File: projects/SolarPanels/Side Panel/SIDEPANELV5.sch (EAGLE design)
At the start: 31 parts

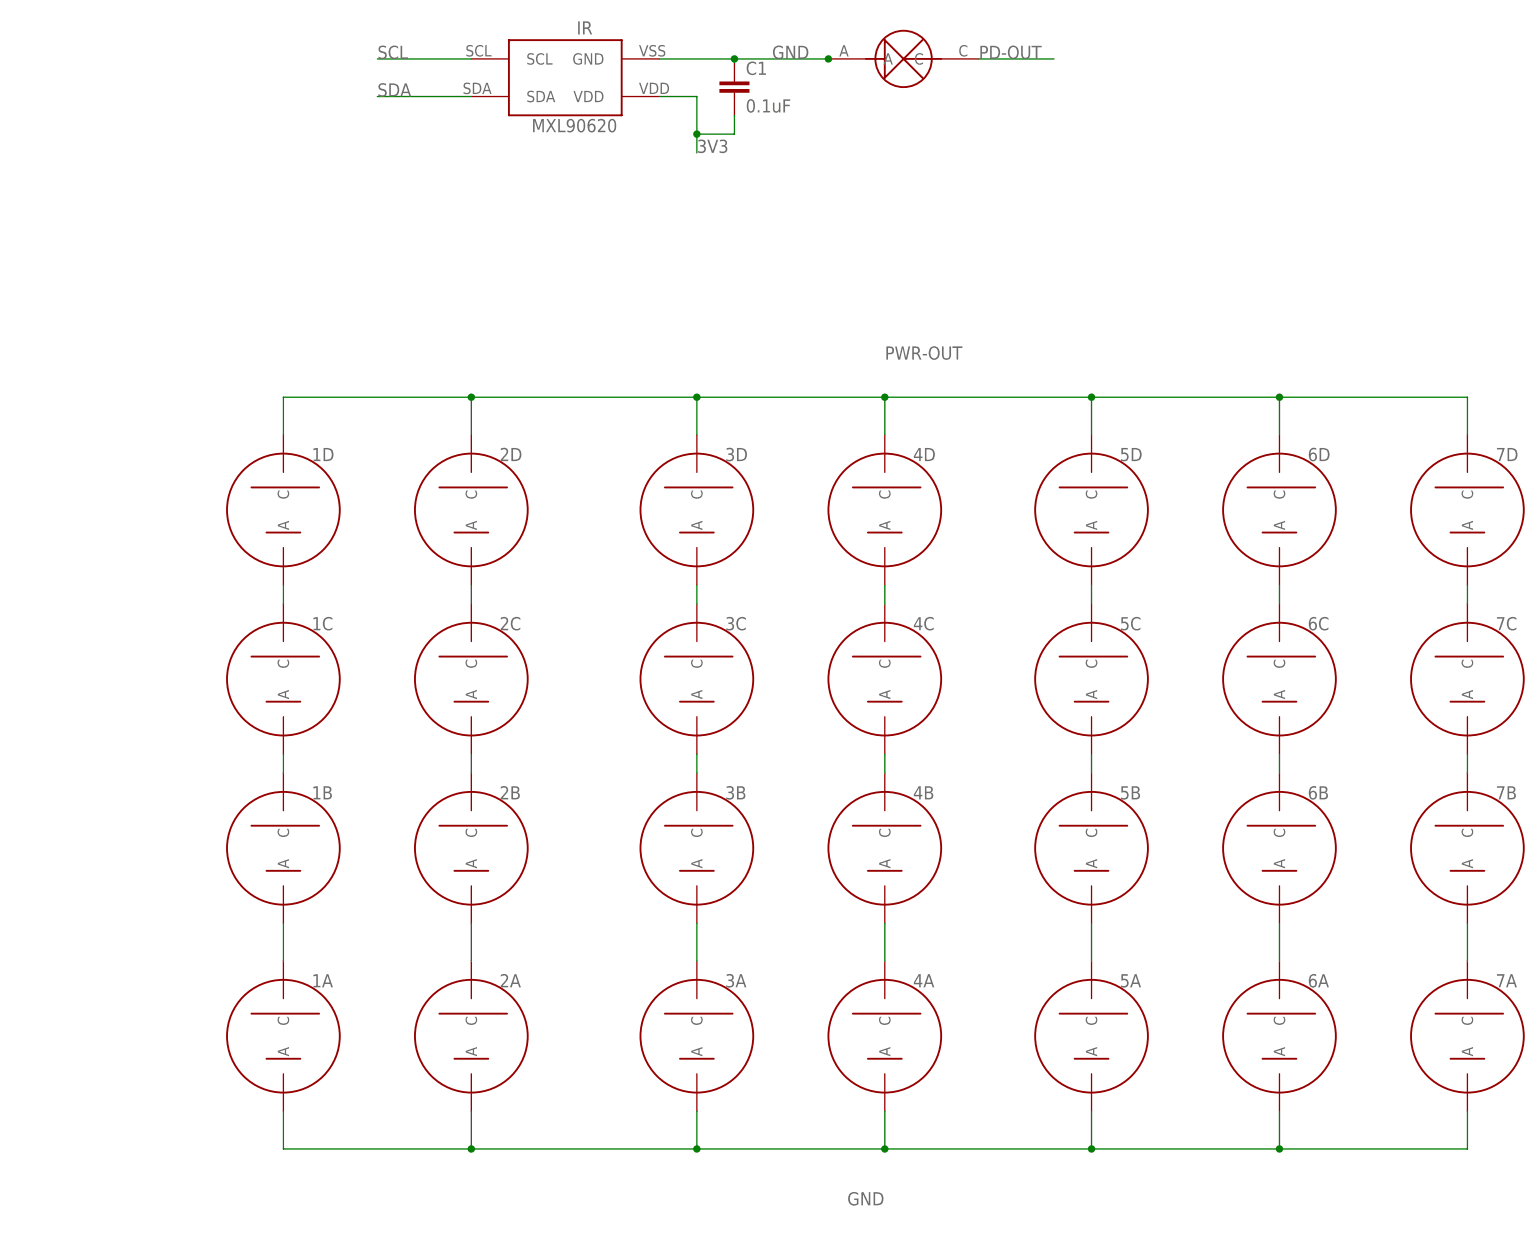
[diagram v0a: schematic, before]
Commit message: Side Panel V5 Finished (?)
Ready to be checked
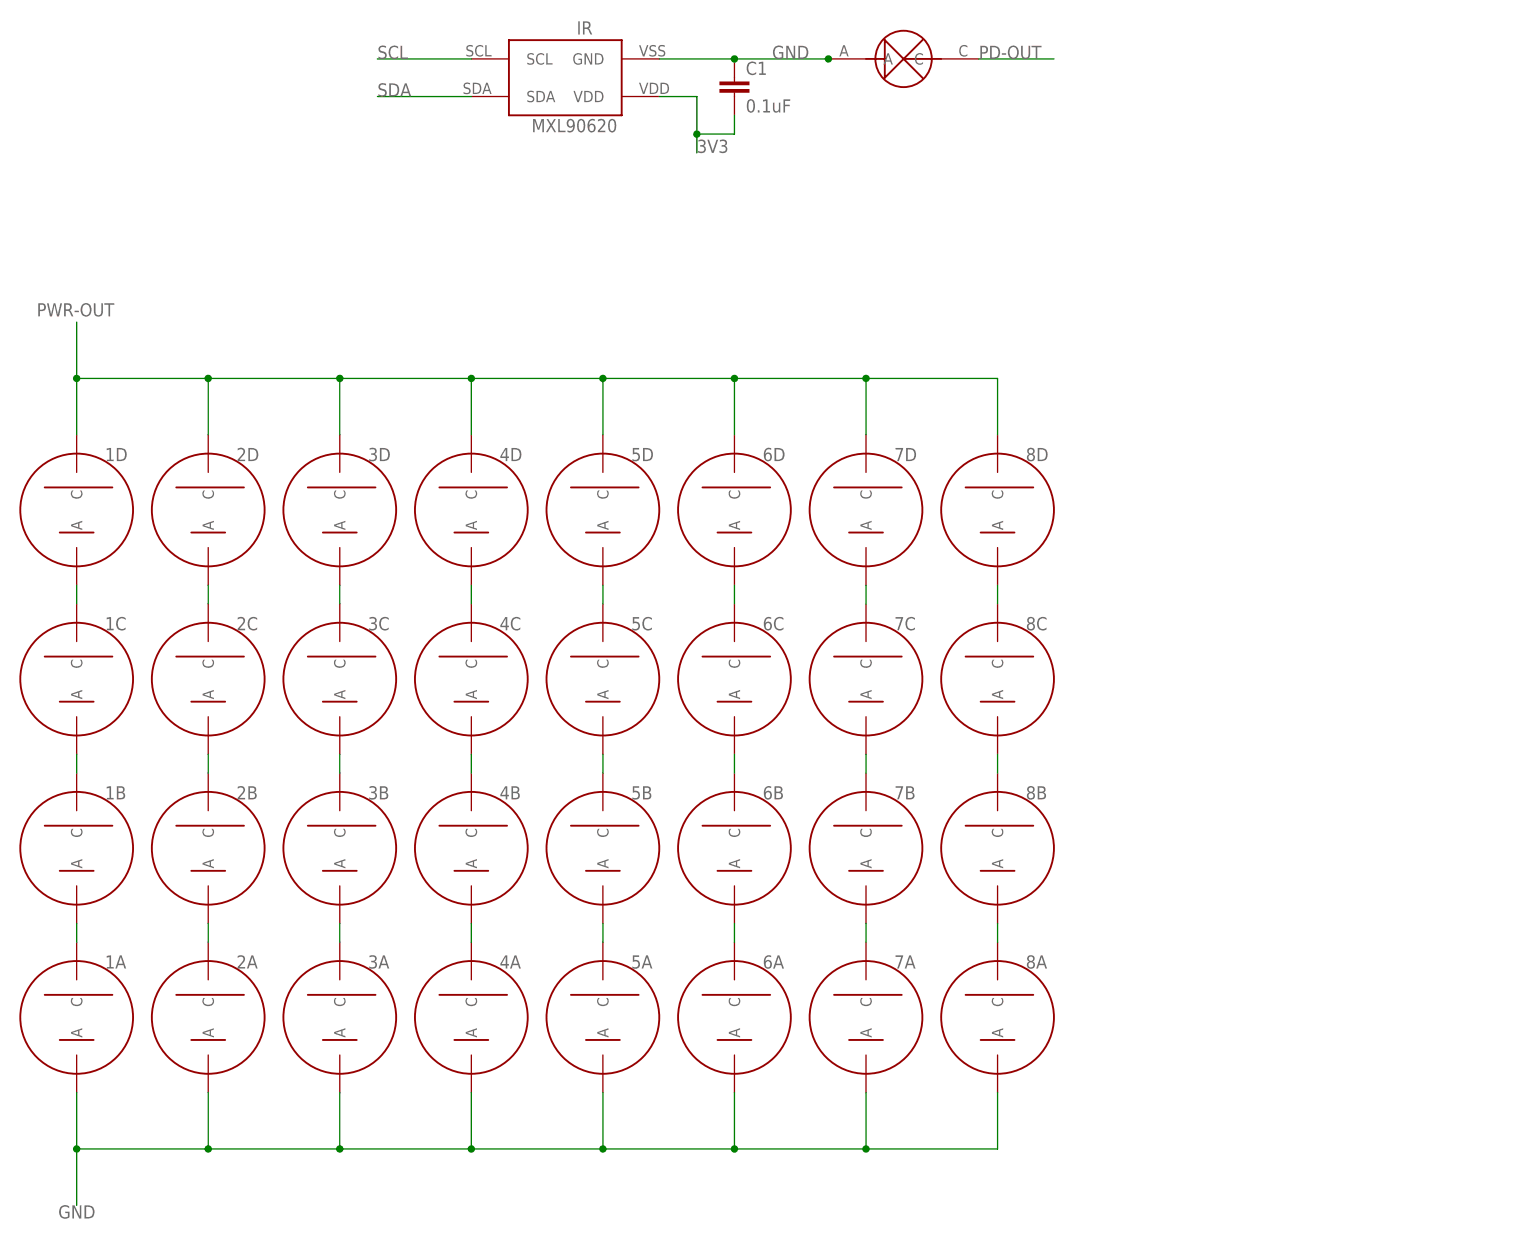
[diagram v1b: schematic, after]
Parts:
- added 8A, 8B, 8C, 8D: SOLARCELLV3, BrownSpaceEngineering:SOLARCELLV3
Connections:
- net 2C renamed N$5
- new net N$23: 8C.C, 8D.A
- new net N$24: 8B.C, 8C.A
- new net N$25: 8A.C, 8B.A
- net GND: now also 8A.A
- net PWR-OUT: now also 8D.C
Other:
- moved on the sheet: 1A, 1B, 1C, 1D, 2A, 2B, 2C, 2D, 3A, 3B, 3C, 3D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
